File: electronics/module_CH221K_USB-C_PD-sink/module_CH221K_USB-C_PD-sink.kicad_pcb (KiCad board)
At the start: 2 copper layers, 23.5 x 18.2 mm, 20 parts, among them J1 USB-C_PD, J2 Conn_01x02, Q1 PMOS, U1 CH221K

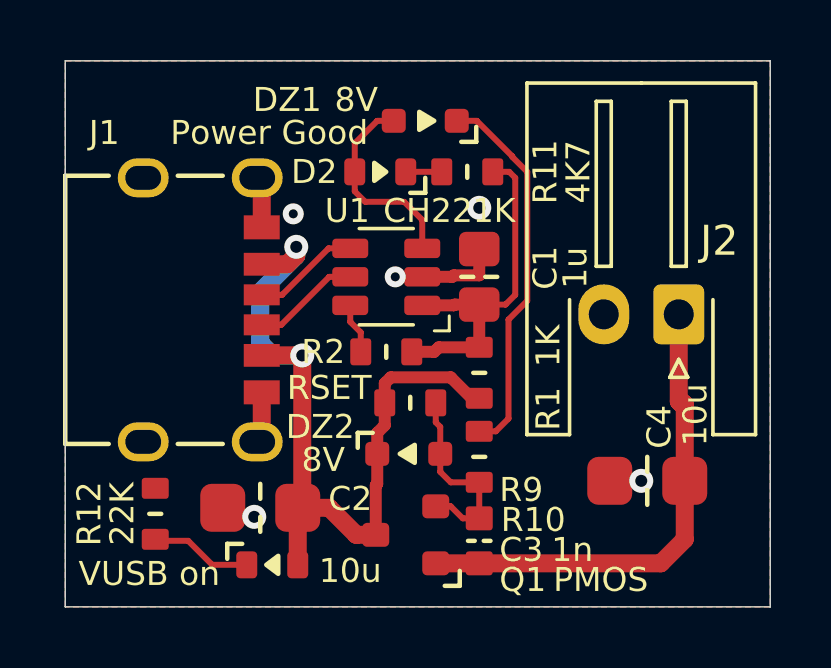
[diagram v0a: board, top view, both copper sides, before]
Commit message: fixed issues and simplified
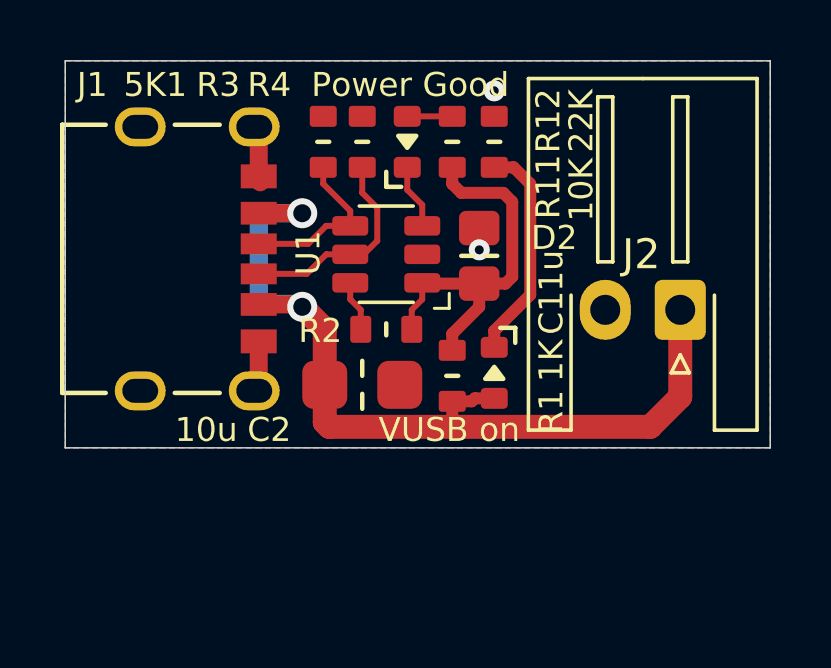
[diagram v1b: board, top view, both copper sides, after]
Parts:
- removed C3: 1n, SquantorCapacitor:C_0603
- removed C4: 10u, SquantorCapacitor:C_1206_0805
- removed DZ1, DZ2: 8V, SquantorDiodes:SOD-323-nexperia-hand
- removed Q1: PMOS, SquantorIC:SOT23-3
- removed R10: PD, SquantorResistor:R_0603_hand
- removed R9: PU, SquantorResistor:R_0603_hand
- added R3: 5K1, SquantorResistor:R_0603_hand, F.Cu at (97.3, 45.8)
- added R4: 5K1, SquantorResistor:R_0603_hand, F.Cu at (98.6, 45.8)
- R11: value 4K7 -> 10K
- moved R12 16.8 mm to (103.0, 45.8)
- moved D3 9.78 mm to (103.0, 53.5), turned to -90 degrees
- moved C2 5.33 mm to (98.6, 53.9), turned to 0 degrees
- moved N1 2.25 mm to (101.0, 53.4)
- moved N2 2.25 mm to (101.8, 49.9)
- moved J1 1.70 mm to (95.2, 49.7)
- moved D2 1.35 mm to (100.1, 45.8), turned to 90 degrees
- moved R11 1.12 mm to (101.6, 45.8), turned to 90 degrees
- moved R1 0.91 mm to (101.6, 53.6)
- moved R2 0.75 mm to (99.4, 52.0)
- moved U1 0.75 mm to (99.4, 49.5)
- moved C1 0.70 mm to (102.5, 49.6)
- moved J2 0.16 mm to (109.2, 51.4)
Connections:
- D2 pad 1: Net-(D2-K) -> /PG
- D2 pad 2: /PG -> Net-(D2-A)
- J2 pad 1: /VOUT -> /VBUS
- R11 pad 2: Net-(D2-K) -> Net-(D2-A)
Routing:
- net /VOUT: track 16.3 -> 0.00 mm
- net Net-(DZ1-K): track 12.7 -> 0.00 mm
- net Net-(DZ2-A): track 6.62 -> 0.00 mm
- net /PG: track 6.80 -> 2.16 mm
- net Net-(D3-K): track 2.98 -> 7.37 mm
- net /VBUS: track 26.9 -> 30.4 mm
- net /CC2: track 3.61 -> 7.06 mm
- net GND: track 6.22 -> 3.42 mm, vias 5 -> 2
- net /CC1: track 3.59 -> 5.62 mm
- net Net-(D2-A): track 0.00 -> 1.50 mm
- net Net-(D2-K): track 1.20 -> 0.00 mm
- net /VDD: track 11.7 -> 12.7 mm
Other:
- board size 23.5 x 18.2 mm -> 23.5 x 12.9 mm
